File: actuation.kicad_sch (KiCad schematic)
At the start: 21 parts, among them J115F? J115F11C24VACS6

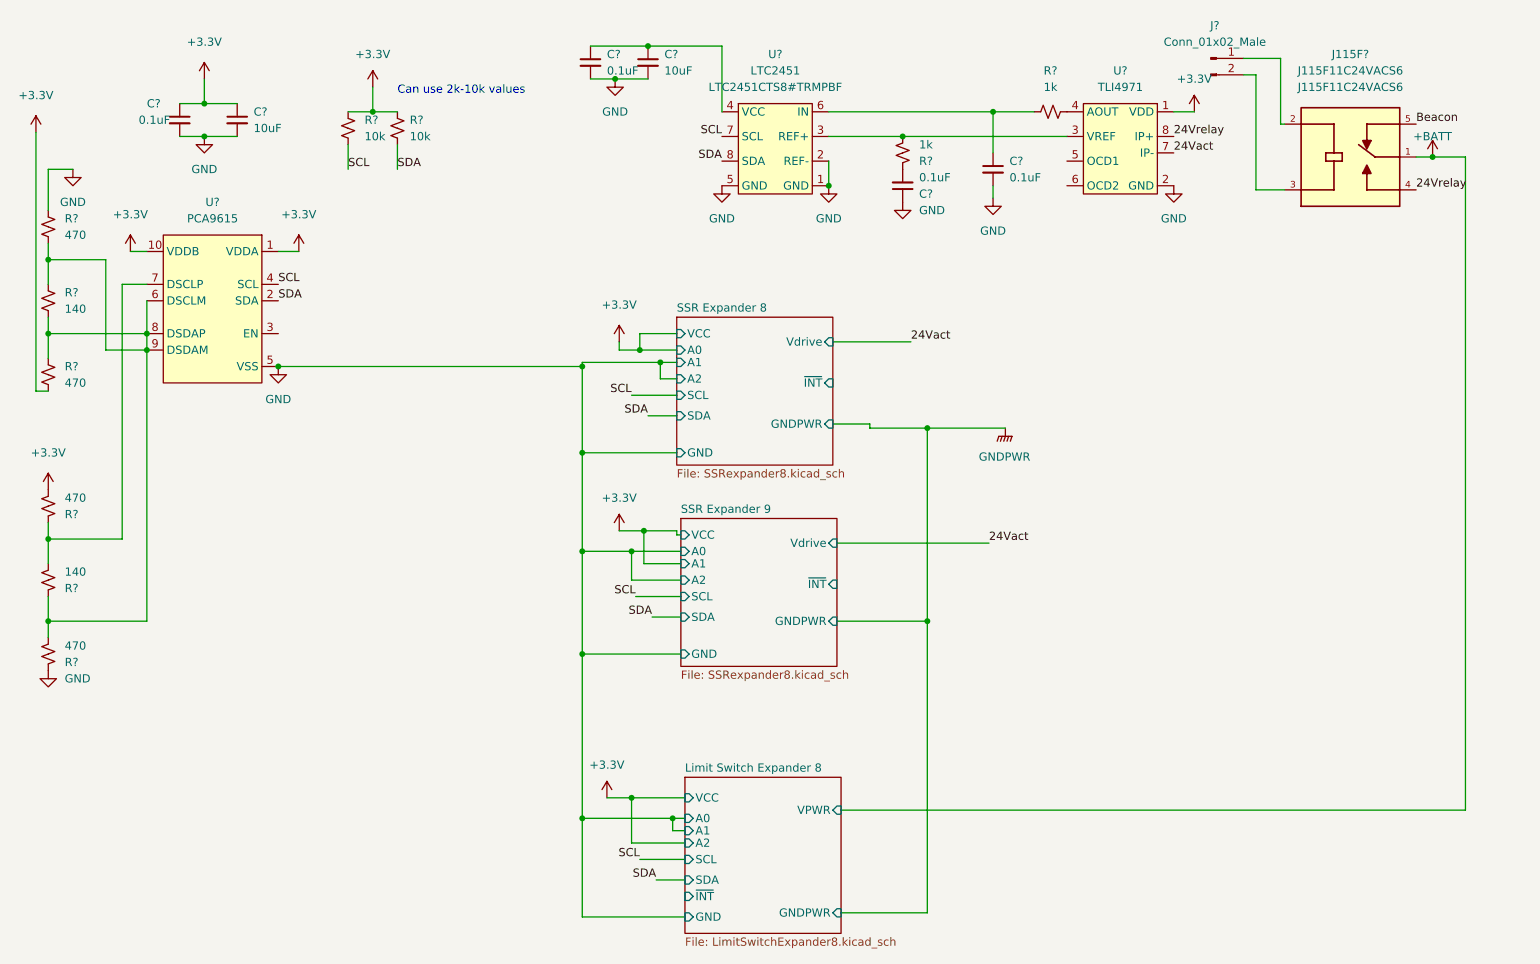
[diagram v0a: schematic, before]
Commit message: Grid issues
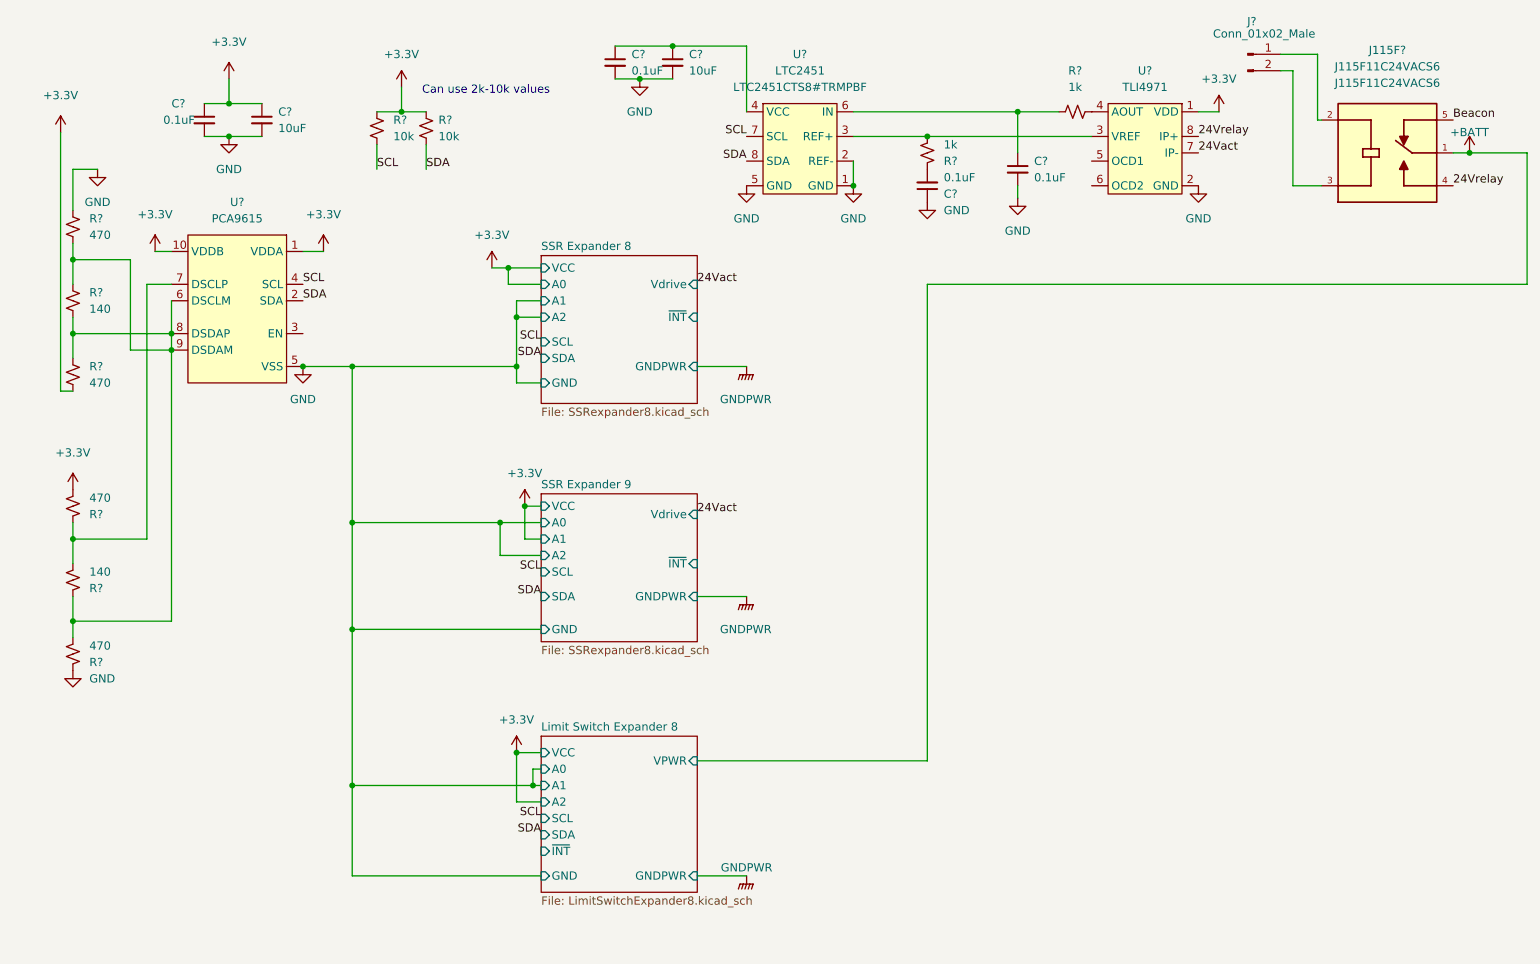
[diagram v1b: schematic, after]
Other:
- moved on the sheet: C?, J115F?, J?, R?, U?
